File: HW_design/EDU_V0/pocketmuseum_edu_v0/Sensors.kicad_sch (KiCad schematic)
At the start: 17 parts, among them Q301 BSS138, Q302 BSS138, Q303 BSS138, U301 ICM-20948, U302 ICP20100

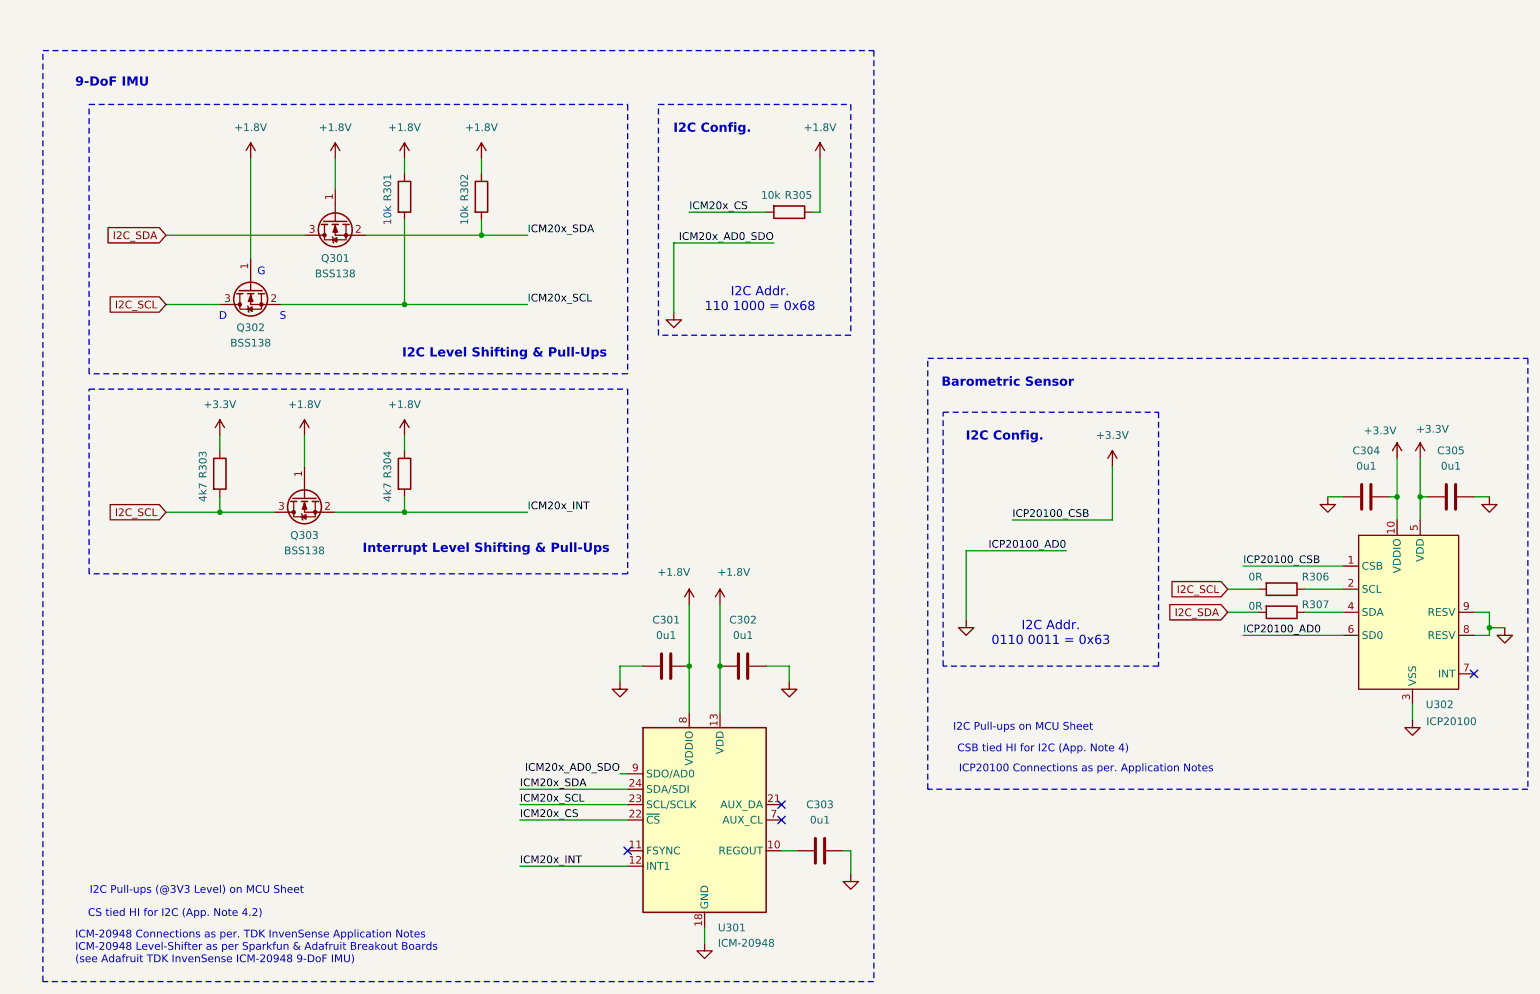
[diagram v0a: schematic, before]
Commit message: Updated Readme
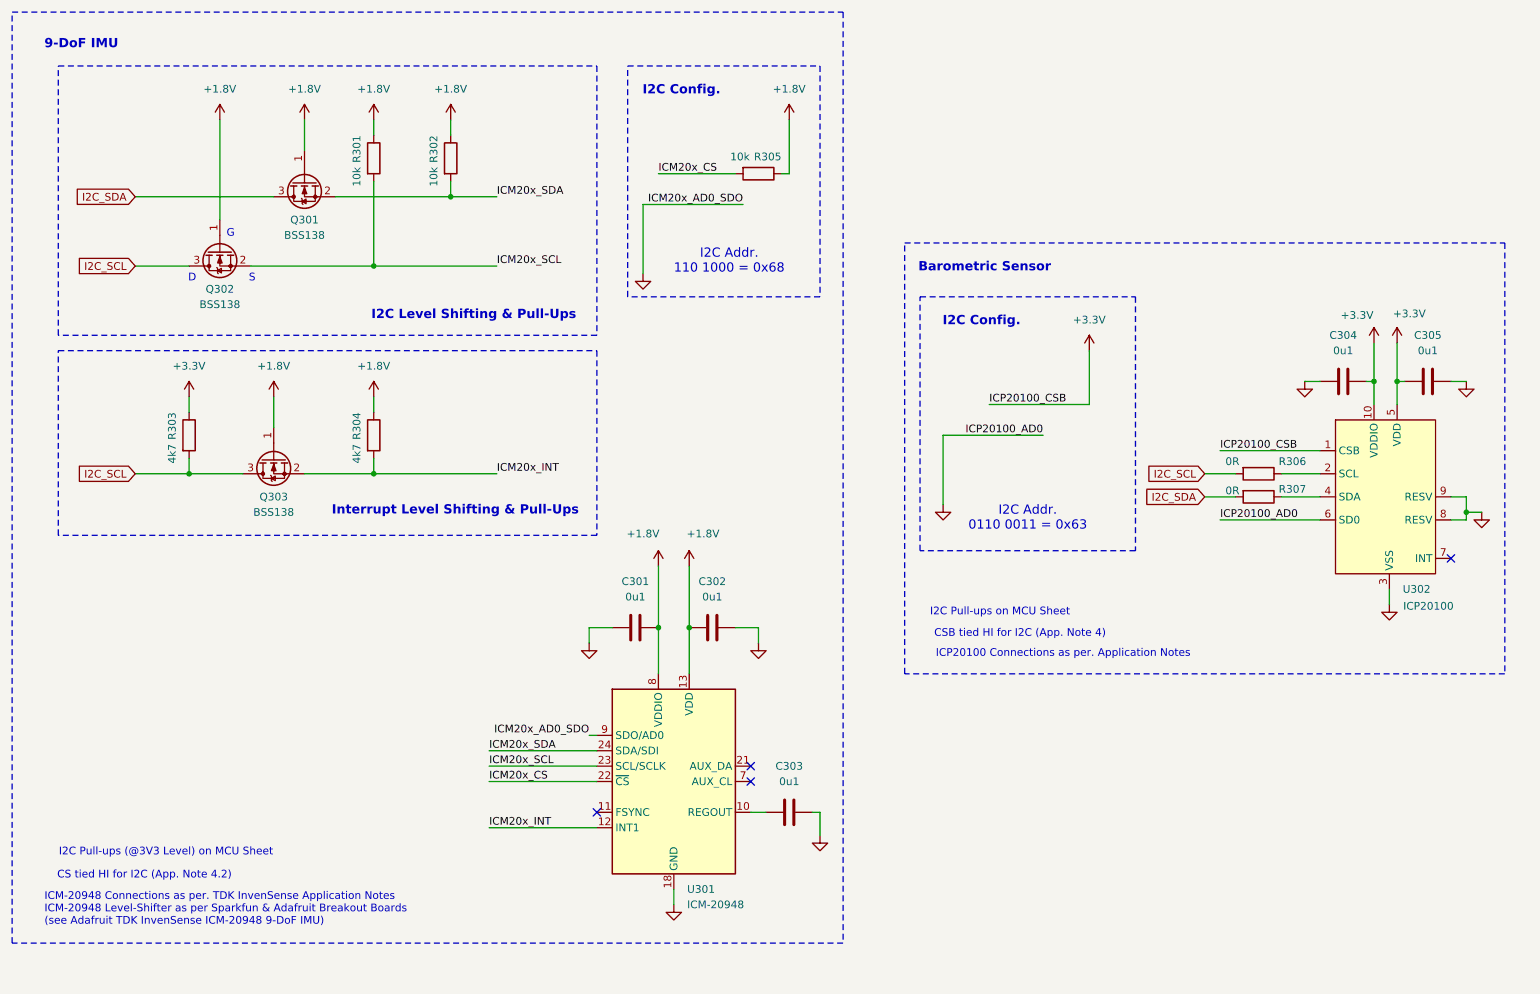
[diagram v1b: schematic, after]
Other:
- company: (none) -> Bucharest Applied STEAM Museum
- title: (none) -> POCKETMUSEUM EDU V0
- moved on the sheet: C301, C302, C303, C304, C305, Q301, Q302, Q303, R301, R302, R303, R304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
